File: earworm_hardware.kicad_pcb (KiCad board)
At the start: 2 copper layers, 37 parts, among them J1 Conn_01x02, J2 Conn_01x05, T1 LPR6235-752SMRC, U1 LTC3108EDE-TRPBF, U2 ADXL367BCCZ-RL7, U3 nRF54L15-QFXX, X1 32MHz

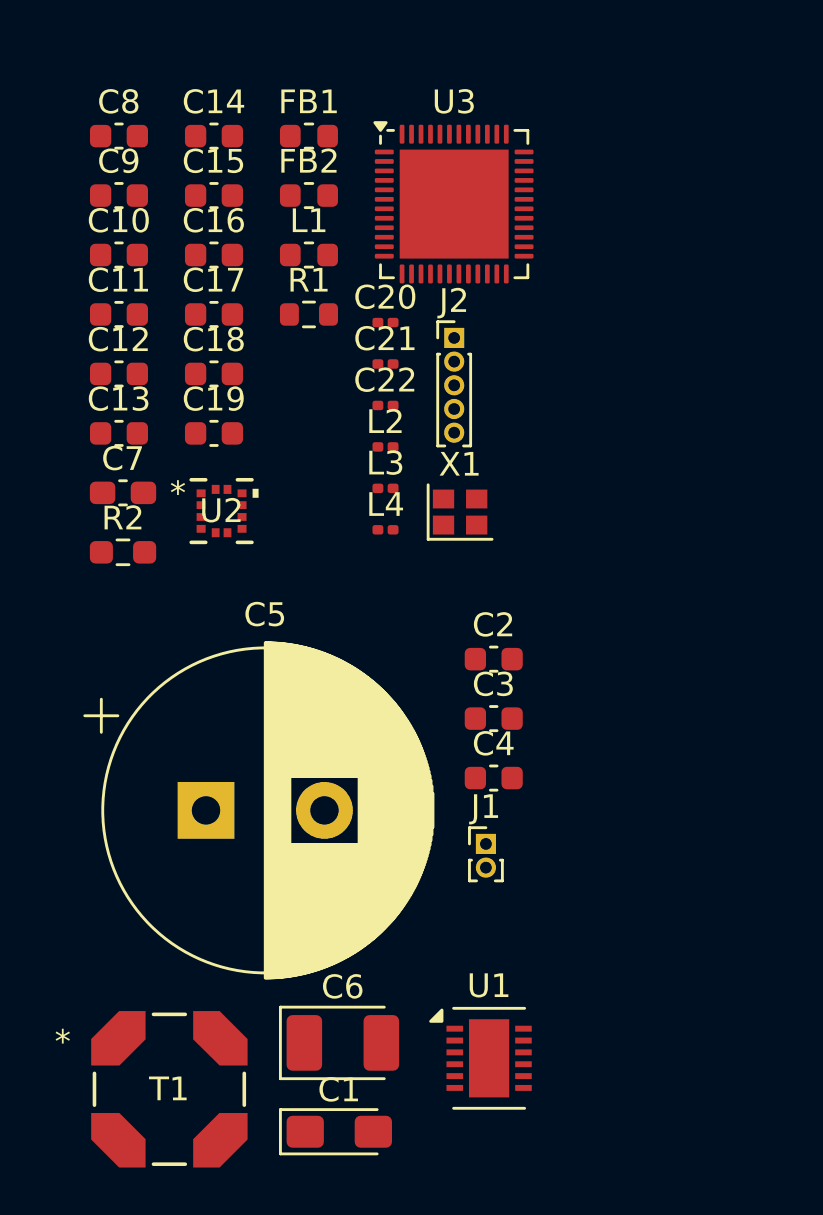
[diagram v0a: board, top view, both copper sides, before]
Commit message: Initial PCB Layout
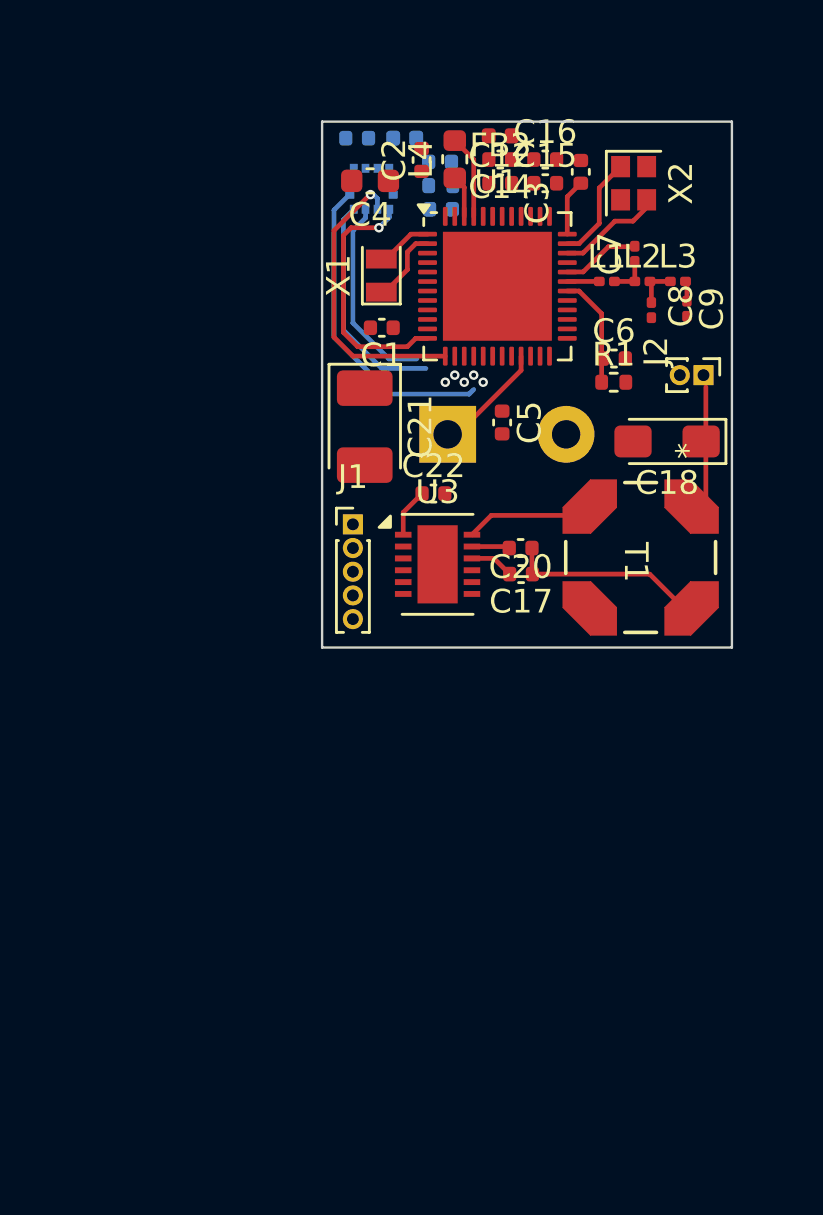
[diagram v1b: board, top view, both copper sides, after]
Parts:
- removed the C11 at (83.0, 82.1)
- added C4: 10uF, Capacitor_SMD:C_0603_1608Metric, F.Cu at (93.6, 76.5)
- added X1: 32.768 kHz, earworm:Crystal_SMD_ECS_2012-2Pin_2.0x1.2mm, F.Cu at (94.1, 80.5)
- C1: renamed from C10; footprint Capacitor_SMD:C_0603_1608Metric -> Capacitor_SMD:C_0402_1005Metric
- C10: renamed from C7; footprint Capacitor_SMD:C_0603_1608Metric_Pad1.08x0.95mm_HandSolder -> Capacitor_SMD:C_0402_1005Metric; moved to B.Cu
- C11: renamed from C9; footprint Capacitor_SMD:C_0603_1608Metric -> Capacitor_SMD:C_0402_1005Metric; moved to B.Cu
- C12: renamed from C15; footprint Capacitor_SMD:C_0603_1608Metric -> Capacitor_SMD:C_0402_1005Metric
- C13: renamed from C8; footprint Capacitor_SMD:C_0603_1608Metric -> Capacitor_SMD:C_0402_1005Metric; moved to B.Cu
- C14: renamed from C16; footprint Capacitor_SMD:C_0603_1608Metric -> Capacitor_SMD:C_0402_1005Metric
- C15: renamed from C18; footprint Capacitor_SMD:C_0603_1608Metric -> Capacitor_SMD:C_0402_1005Metric
- C16: renamed from C19; footprint Capacitor_SMD:C_0603_1608Metric -> Capacitor_SMD:C_0402_1005Metric
- C17: renamed from C2; footprint Capacitor_SMD:C_0603_1608Metric -> Capacitor_SMD:C_0402_1005Metric
- C19: renamed from C5; moved to B.Cu
- C2: renamed from C12; footprint Capacitor_SMD:C_0603_1608Metric -> Capacitor_SMD:C_0402_1005Metric
- C20: renamed from C3; footprint Capacitor_SMD:C_0603_1608Metric -> Capacitor_SMD:C_0402_1005Metric
- C22: renamed from C4; footprint Capacitor_SMD:C_0603_1608Metric -> Capacitor_SMD:C_0402_1005Metric
- C3: renamed from C14; footprint Capacitor_SMD:C_0603_1608Metric -> Capacitor_SMD:C_0402_1005Metric
- C5: renamed from C13; footprint Capacitor_SMD:C_0603_1608Metric -> Capacitor_SMD:C_0402_1005Metric
- C6: renamed from C17; footprint Capacitor_SMD:C_0603_1608Metric -> Capacitor_SMD:C_0402_1005Metric
- FB1: footprint Inductor_SMD:L_0603_1608Metric -> Inductor_SMD:L_0402_1005Metric; moved to B.Cu
- FB2: footprint Inductor_SMD:L_0603_1608Metric -> Inductor_SMD:L_0402_1005Metric
- R1: renamed from R2; footprint Resistor_SMD:R_0603_1608Metric_Pad0.98x0.95mm_HandSolder -> Resistor_SMD:R_0402_1005Metric
- R2: renamed from R1; footprint Resistor_SMD:R_0603_1608Metric -> Resistor_SMD:R_0402_1005Metric; moved to B.Cu
- U2: moved to B.Cu
- moved C18 32.3 mm to (106.2, 87.5), turned to 180 degrees
- moved T1 30.0 mm to (105.0, 92.4), turned to -90 degrees
- moved C21 26.0 mm to (93.4, 86.9), turned to -90 degrees
- moved R1 21.9 mm to (103.9, 85.0)
- moved J2 21.8 mm to (107.7, 84.7), turned to -90 degrees
- moved U3 21.0 mm to (96.5, 92.7)
- moved C10 19.3 mm to (96.6, 75.7)
- moved C19 18.9 mm to (96.9, 87.2)
- moved C16 18.1 mm to (101.0, 75.6)
- moved C6 17.0 mm to (103.9, 84.0)
- moved L3 16.2 mm to (106.6, 80.7)
- moved C5 16.2 mm to (99.2, 86.7), turned to -90 degrees
- moved C15 16.1 mm to (101.0, 76.6)
- moved X2 15.7 mm to (104.8, 76.6), turned to -90 degrees
- moved C2 15.6 mm to (95.8, 75.6), turned to 90 degrees
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- renumbered C1 to C18, C6 to C21, C20 to C7, C21 to C8, C22 to C9, J2 to J1, J1 to J2, L2 to L1, L3 to L2, L4 to L3, L1 to L4, U3 to U1, U1 to U3, X1 to X2
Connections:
- U1 pad 1: unconnected-(U3-P1.00-Pad1) -> Net-(U1-P1.00)
- U1 pad 2: unconnected-(U3-P1.01-Pad2) -> Net-(U1-P1.01)
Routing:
- net Net-(U1-P2.05): track 0.00 -> 13.3 mm
- net Net-(U1-P2.02): track 0.00 -> 12.5 mm, vias 0 -> 1
- net Net-(U1-P2.01): track 0.00 -> 10.6 mm, vias 0 -> 1
- net Net-(U1-P2.04): track 0.00 -> 9.43 mm
- net Net-(T1-SB): track 0.00 -> 8.52 mm
- net Net-(U1-P2.03): track 0.00 -> 8.35 mm
- net Net-(J2-Pin_1): track 0.00 -> 5.71 mm
- net Net-(T1-AB): track 0.00 -> 5.36 mm
- net /Thermal Energy Harvesting Chain/VSTORE: track 0.00 -> 5.22 mm
- net Net-(U1-~{RESET}): track 0.00 -> 4.74 mm
- net Net-(U1-XC2): track 0.00 -> 4.47 mm
- net Net-(U1-XC1): track 0.00 -> 4.47 mm
- net Net-(U1-P1.01): track 0.00 -> 3.48 mm
- net GND: track 0.00 -> 3.30 mm
- net Net-(U1-DECD): track 0.00 -> 3.11 mm
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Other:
- board outline added: 17.3 x 22.2 mm
- board text added: "EECS 598 EARWORM"

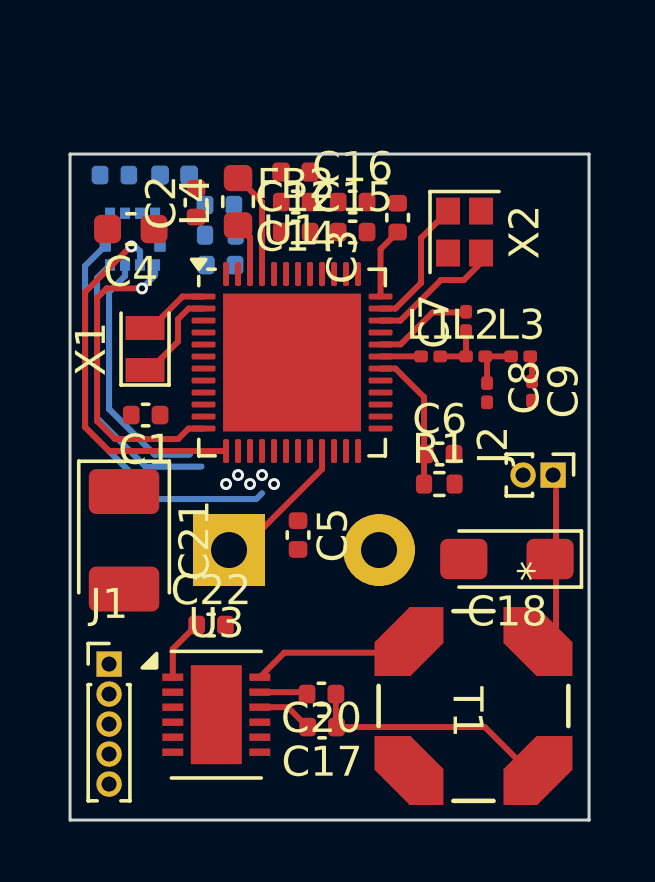
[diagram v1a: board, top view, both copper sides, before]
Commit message: Initial RF layout
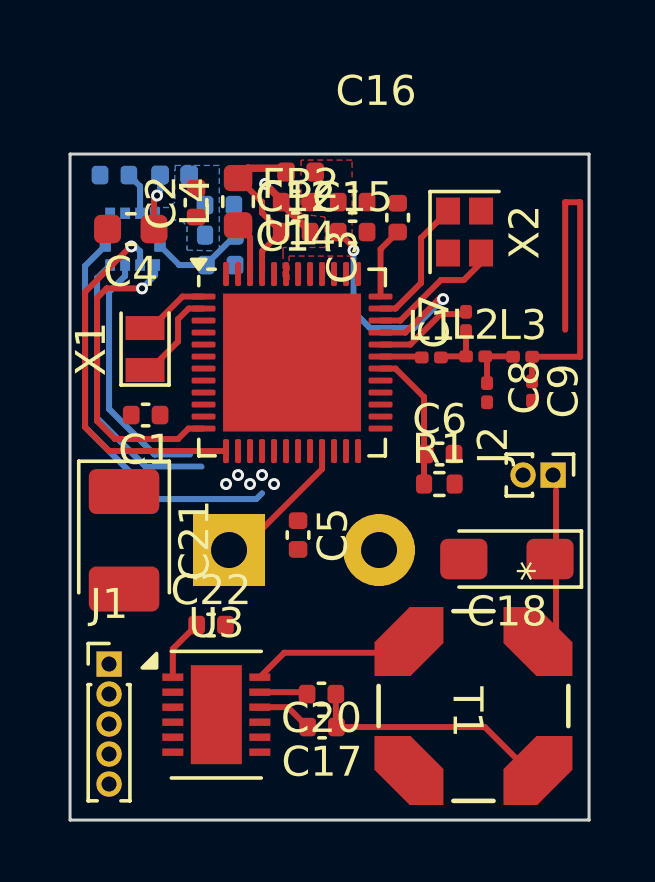
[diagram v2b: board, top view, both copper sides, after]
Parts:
- moved FB2 0.16 mm to (99.3, 74.6)
- moved L3 0.07 mm to (106.7, 80.8)
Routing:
- net Net-(U1-DECA): track 0.00 -> 9.02 mm, vias 0 -> 2
- net Net-(U2-VDDIO): track 0.00 -> 3.20 mm
- net Net-(U1-DECD): track 3.11 -> 5.85 mm
- net GND: track 3.30 -> 5.55 mm, vias 0 -> 1
- net VDD: track 2.39 -> 4.27 mm, vias 0 -> 1
- net Net-(U2-VREG_OUT): track 0.00 -> 1.43 mm
- added copper zone on B.Cu, net GND
- added copper zone on F.Cu, net Net-(U1-DECA)
- added copper zone on B.Cu, net Net-(U2-VS)

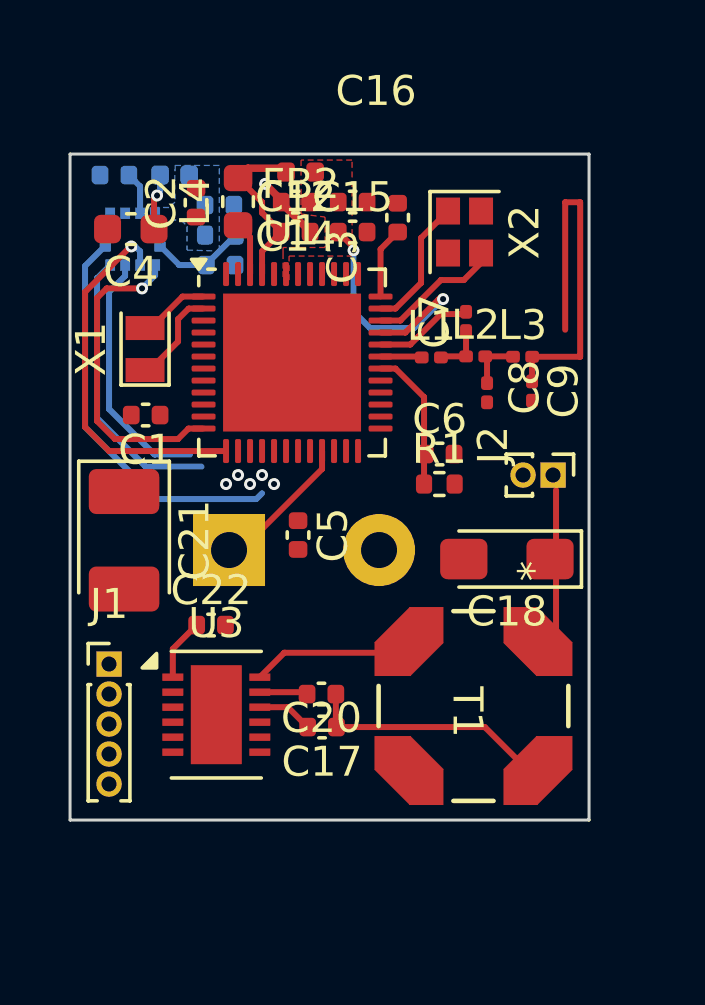
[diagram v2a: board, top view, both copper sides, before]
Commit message: DRC passed, everything done except RF
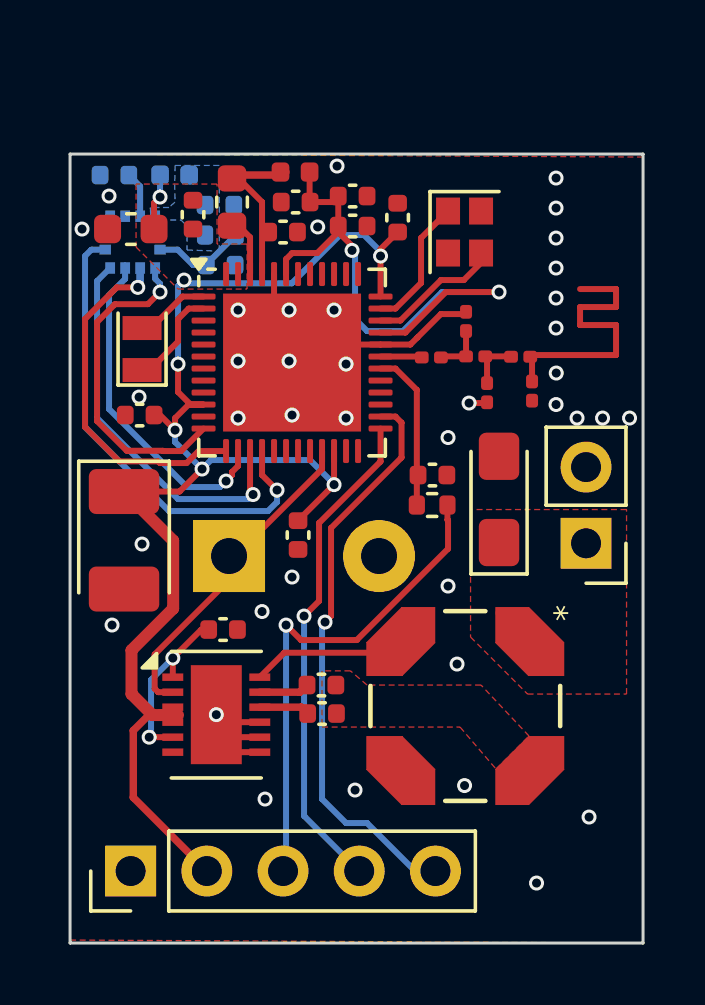
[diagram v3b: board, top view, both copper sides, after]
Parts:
- J1: footprint Connector_PinHeader_1.00mm:PinHeader_1x05_P1.00mm_Vertical -> Connector_PinHeader_2.54mm:PinHeader_1x05_P2.54mm_Vertical
- J2: footprint Connector_PinHeader_1.00mm:PinHeader_1x02_P1.00mm_Vertical -> Connector_PinHeader_2.54mm:PinHeader_1x02_P2.54mm_Vertical
- moved J1 6.94 mm to (93.6, 97.9), turned to 90 degrees
- moved J2 2.53 mm to (108.8, 87.0), turned to 180 degrees
- moved C18 2.00 mm to (105.9, 85.5), turned to 90 degrees
- moved C6 0.74 mm to (103.7, 84.7)
- moved R1 0.74 mm to (103.7, 85.7)
- moved C17 0.45 mm to (100.0, 92.7)
- moved C22 0.43 mm to (96.7, 89.8)
- moved C12 0.42 mm to (98.7, 76.6)
- moved C2 0.41 mm to (95.7, 76.0)
- moved C20 0.30 mm to (100.0, 91.7)
- moved T1 0.27 mm to (104.8, 92.4)
- moved L4 0.20 mm to (97.0, 75.6)
- moved C1 0.20 mm to (93.9, 82.7)
- moved C19 0.20 mm to (96.9, 87.4)
- moved C15 0.20 mm to (101.0, 76.4)
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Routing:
- net VDD: track 4.27 -> 47.7 mm, vias 1 -> 7
- net /nRF54L15 RFSoC/SWCLK: track 0.00 -> 19.2 mm, vias 0 -> 1
- net /nRF54L15 RFSoC/NRST: track 0.00 -> 16.6 mm, vias 0 -> 1
- net /nRF54L15 RFSoC/SWDIO: track 0.00 -> 16.6 mm, vias 0 -> 1
- net Net-(U1-DECA): track 9.02 -> 18.7 mm
- net GND: track 5.55 -> 14.6 mm, vias 1 -> 39
- net Net-(T1-SB): track 8.52 -> 0.00 mm
- net /Thermal Energy Harvesting Chain/VSTORE: track 5.22 -> 11.5 mm
- net Net-(J2-Pin_1): track 5.71 -> 1.70 mm
- net Net-(U3-VAUX): track 2.07 -> 5.98 mm, vias 0 -> 2
- net Net-(U1-P2.04): track 9.43 -> 13.1 mm, vias 0 -> 1
- net Net-(U1-P2.03): track 8.35 -> 11.2 mm, vias 0 -> 1
- net Net-(U1-P2.05): track 13.3 -> 16.1 mm, vias 0 -> 1
- net Net-(U1-P2.02): track 12.5 -> 11.8 mm
- net Net-(U1-DECD): track 5.85 -> 5.21 mm
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- added copper zone on F.Cu, net GND
- added copper zone on F.Cu, net Net-(J2-Pin_1)
- added copper zone on F.Cu, net Net-(T1-SB)
- added copper zone on F.Cu, net VDD
- removed copper zone on F.Cu, net Net-(U1-DECA)
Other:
- board size 17.3 x 22.2 mm -> 19.1 x 26.3 mm
